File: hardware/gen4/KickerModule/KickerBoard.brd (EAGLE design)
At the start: 317.6 x 151.4 mm, 119 parts

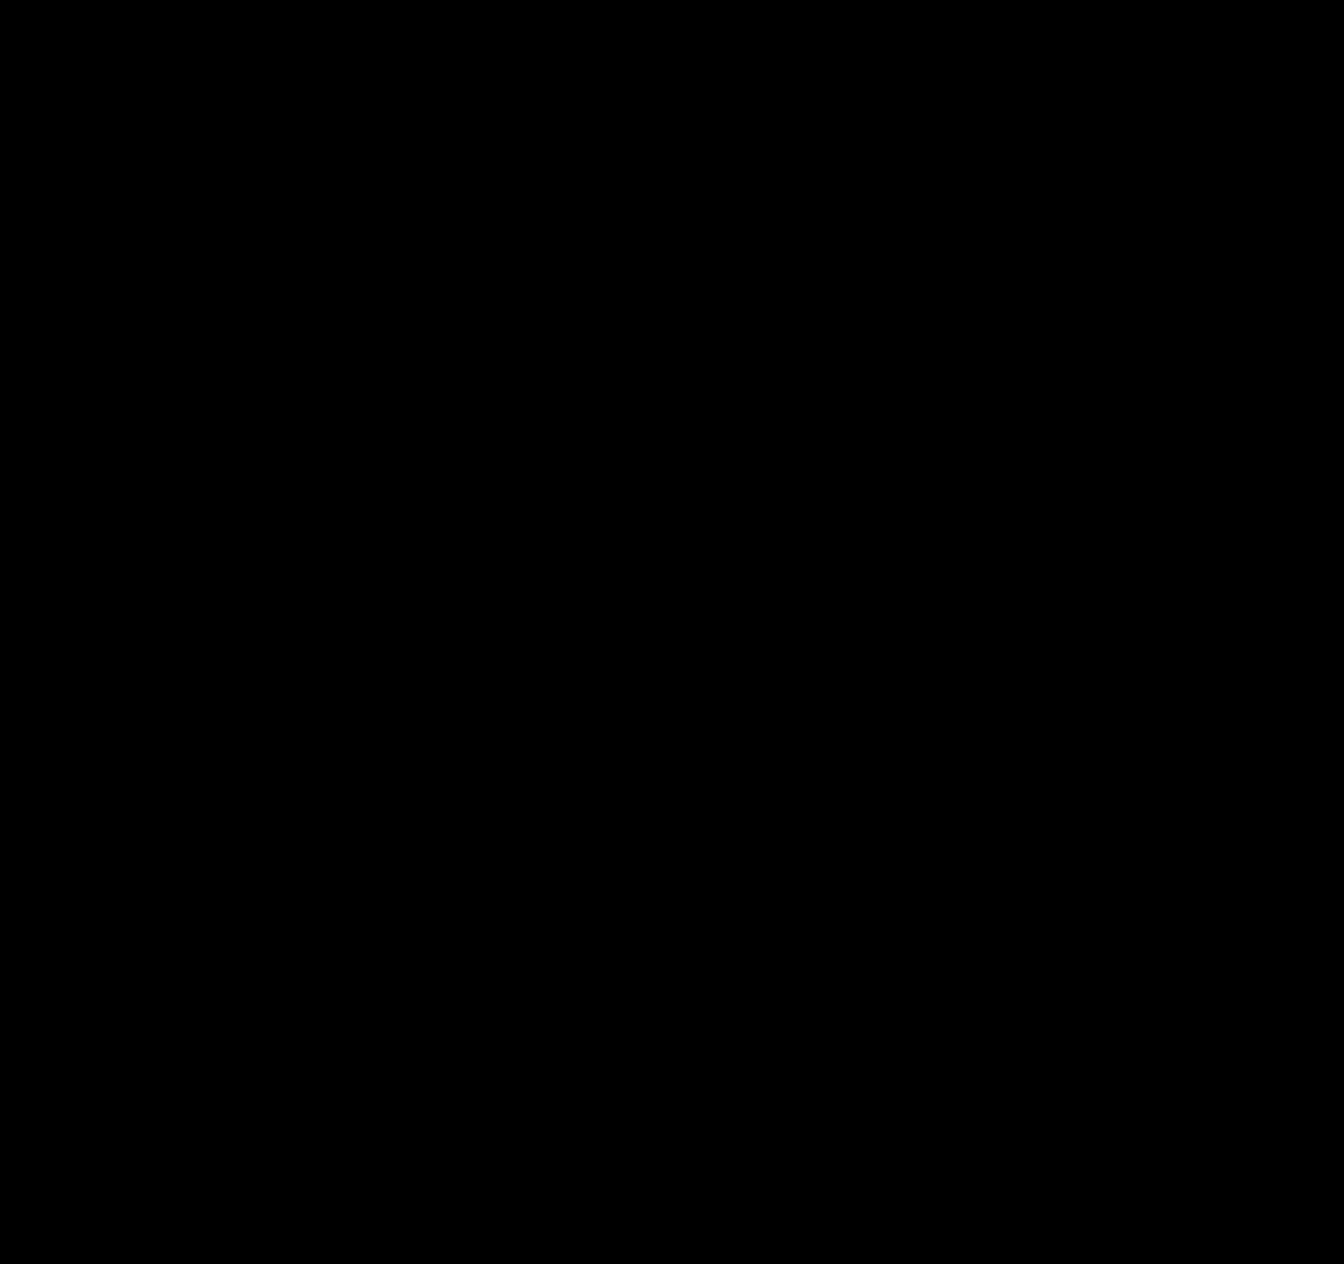
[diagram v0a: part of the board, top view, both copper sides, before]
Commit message: new shape
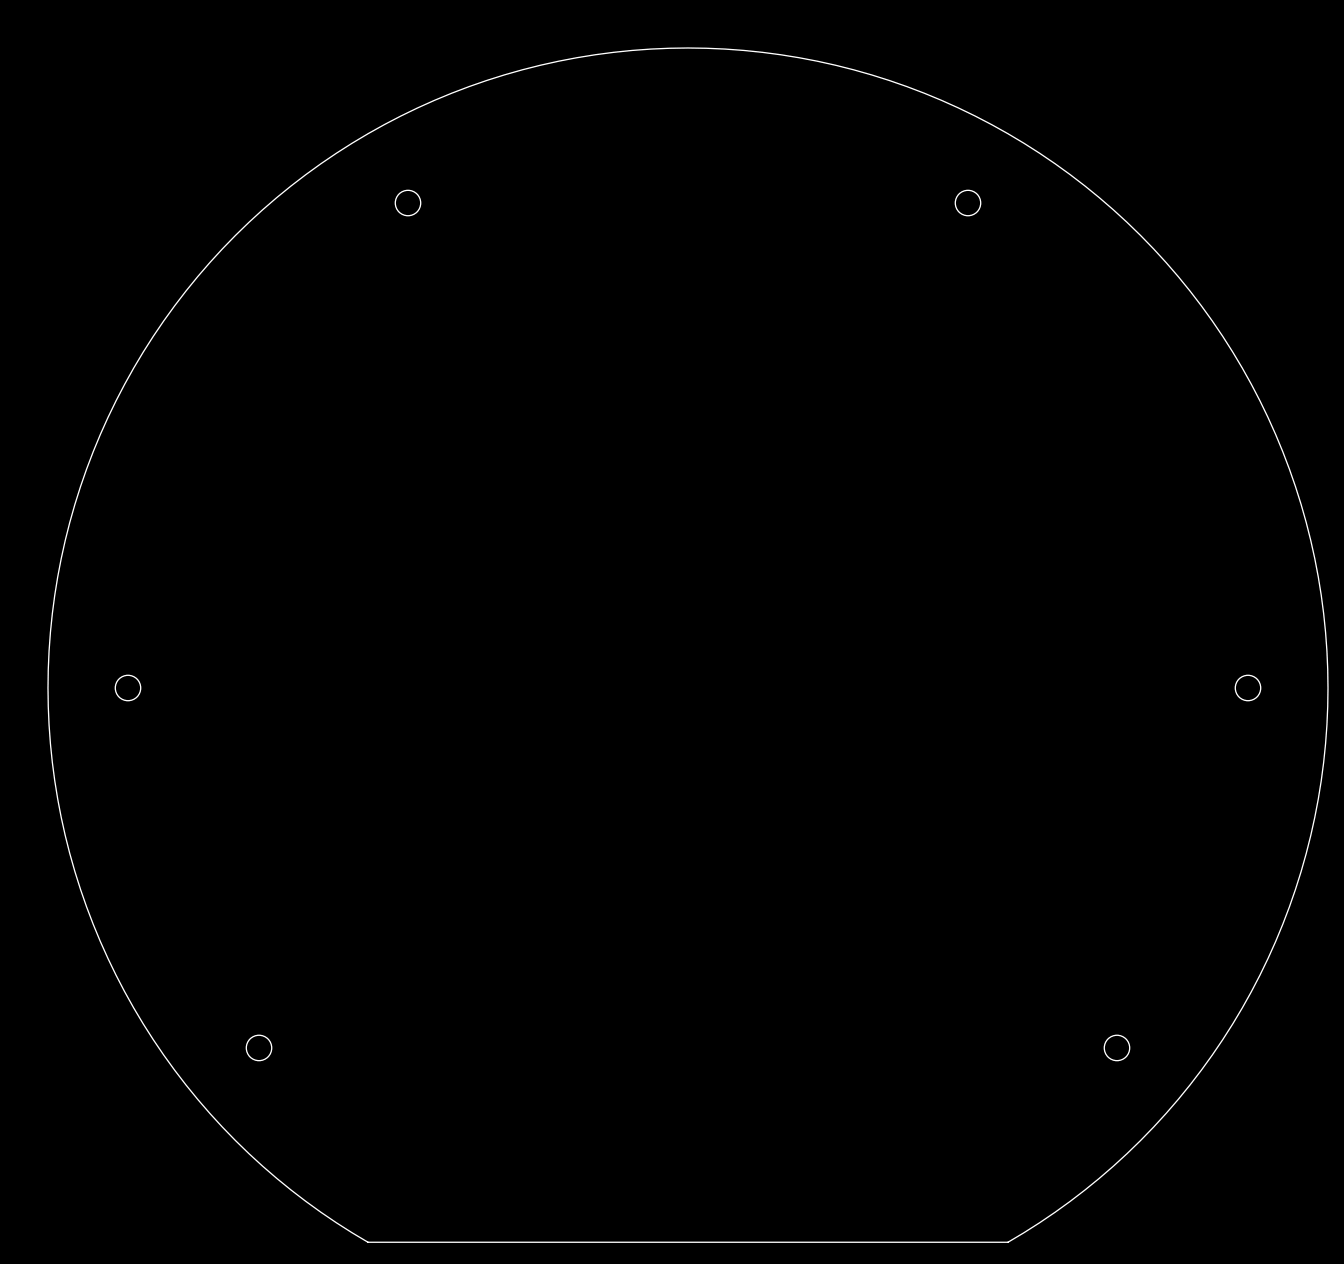
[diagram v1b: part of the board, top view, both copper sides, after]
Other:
- board size 317.6 x 151.4 mm -> 513.1 x 154.5 mm
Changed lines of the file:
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@@
 <wire x1="-33.544509375" y1="112.649253125" x2="-71.0445625" y2="150.14930625" width="0" layer="20"/>
 <wire x1="-33.544509375" y1="42.649140625" x2="-33.544509375" y2="112.649253125" width="0" layer="20"/>
+<circle x="324.508875" y="64.897" radius="1.5875" width="0" layer="20"/>
+<circle x="184.508903125" y="64.897" radius="1.5875" width="0" layer="20"/>
+<circle x="219.50883125" y="125.518671875" radius="1.5875" width="0" layer="20"/>
+<circle x="289.508690625" y="125.518671875" radius="1.5875" width="0" layer="20"/>
+<circle x="308.131971875" y="19.901915625" radius="1.5875" width="0" layer="20"/>
+<circle x="200.88580625" y="19.901915625" radius="1.5875" width="0" layer="20"/>
+<wire x1="294.50868125" y1="-4.38505625" x2="214.508840625" y2="-4.38505625" width="0" layer="20"/>
+<wire x1="294.50868125" y1="-4.38505625" x2="214.508840625" y2="-4.38505625" width="0" layer="20" curve="300.000116"/>
 </plain>
 <attributes>

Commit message: new shape part2
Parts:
- moved DRIB 13.3 mm to (26.0, 16.5)
- moved DRIB_TRAN 10.3 mm to (21.0, 21.0), flipped to the bottom
- moved BB_CON 8.28 mm to (38.1, 10.8)
- moved R25 8.25 mm to (41.3, 141.6)
- moved R13 6.99 mm to (37.5, 142.2)
- moved R16 6.99 mm to (37.5, 140.3)
- moved R3 6.99 mm to (37.5, 138.4)
- moved U$6 6.98 mm to (41.3, 146.1)
- moved DRIB_TEST 6.35 mm to (30.5, 9.53)
- moved C12 6.02 mm to (34.3, 13.3), flipped to the bottom
- moved R19 6.02 mm to (36.8, 13.3), flipped to the bottom
- moved R20 5.72 mm to (41.3, 13.3), flipped to the bottom
- moved CHARGE_D 4.44 mm to (18.4, 121.9)
- moved U$2 3.86 mm to (43.8, 131.4)
- moved U$7 3.18 mm to (16.5, 128.9)
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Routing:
- net SS1: track 121.2 -> 0.00 mm, vias 2 -> 0
- net BB_OUT: track 75.5 -> 0.00 mm, vias 2 -> 0
- net BB_IN: track 70.0 -> 0.00 mm
- net DRIB: track 69.6 -> 0.00 mm, vias 1 -> 0
- net GND: track 808.5 -> 755.3 mm, vias 31 -> 29
- net 3.3V: track 524.2 -> 504.4 mm, vias 16 -> 15
- net 12VGND: track 702.7 -> 684.0 mm
- net 12V: track 475.8 -> 461.3 mm
- net TO_DRIB: track 9.10 -> 0.00 mm
- net DIVCAP: track 121.7 -> 116.4 mm
- net TRANS_OUT: track 9.38 -> 4.94 mm
- net N$32: track 4.40 -> 0.00 mm
- net N$40: track 4.26 -> 0.00 mm
- net N$36: track 9.75 -> 13.9 mm
- net N$29: track 26.7 -> 29.2 mm
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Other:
- board size 513.1 x 154.5 mm -> 328.9 x 149.3 mm
